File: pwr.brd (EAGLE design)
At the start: 70.3 x 58 mm, 40 parts, among them Q1 IPD65R600C6, T1 750811647, U1 UCC28700

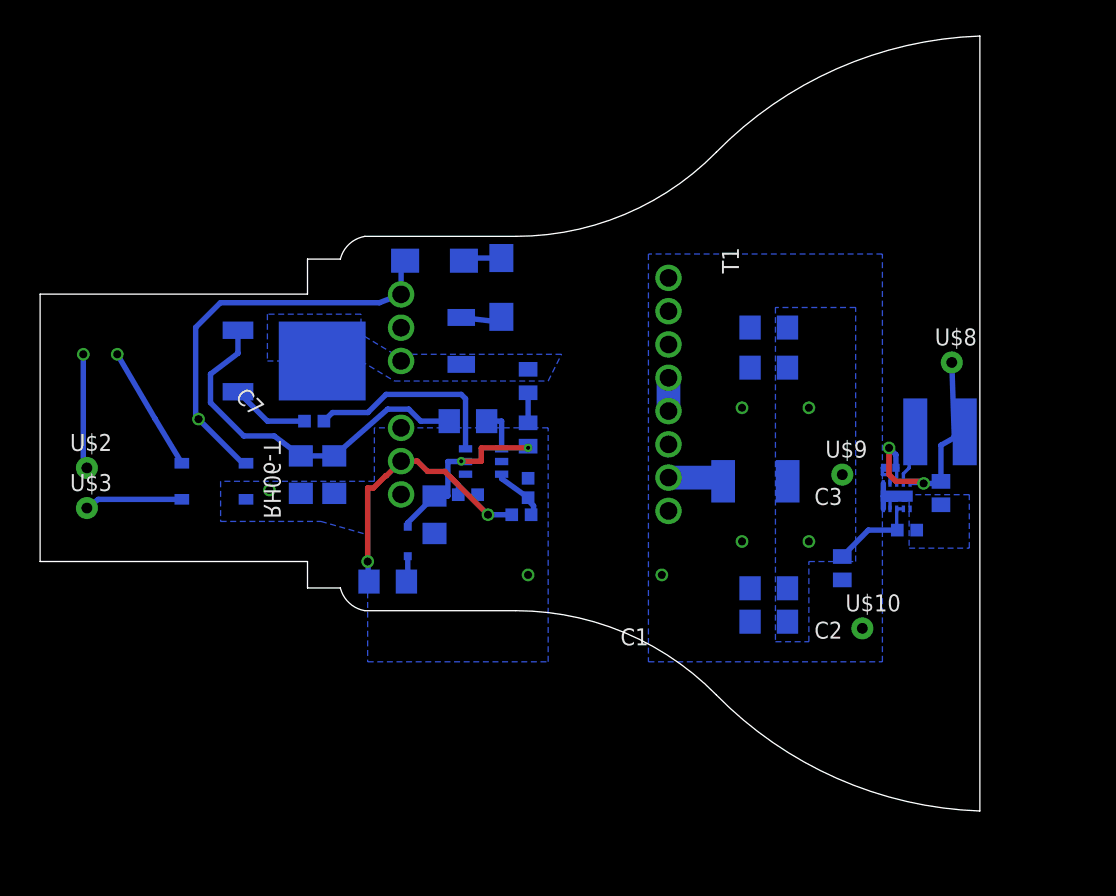
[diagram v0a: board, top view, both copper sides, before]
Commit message: save
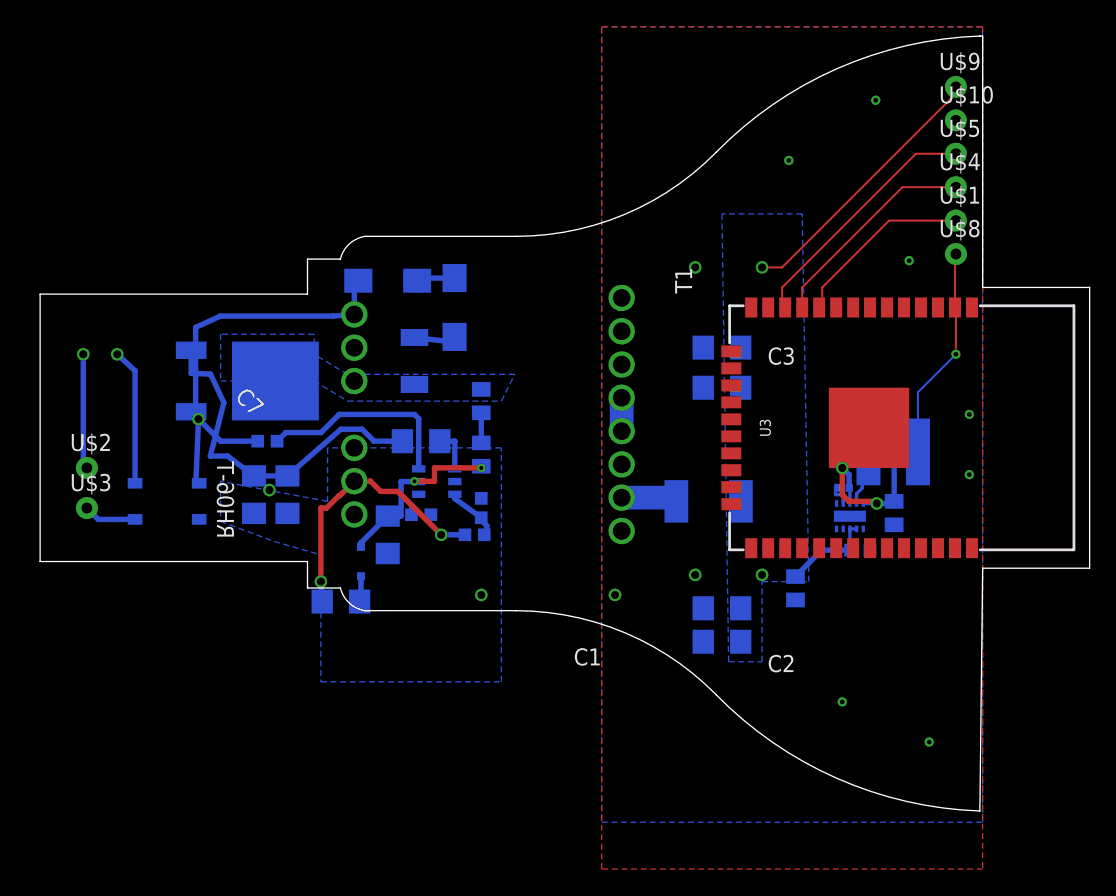
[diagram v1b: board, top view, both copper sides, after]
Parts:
- added U$1, U$4, U$5: TP-1502, derek:TP-1502
- added U3: ESP-WROOM-32, derek:ESP-WROOM-32
- moved U$10 38.6 mm to (74.0, 67.5)
- moved U$9 30.2 mm to (74.0, 70.0)
- moved C3 11.1 mm to (57.0, 56.5)
- moved U$8 8.12 mm to (74.0, 57.5)
- moved C2 4.30 mm to (57.0, 33.5)
- moved C1 3.81 mm to (43.5, 32.0)
- moved C4 3.81 mm to (56.5, 47.5)
- moved C5 3.81 mm to (56.5, 50.5)
- moved C6 3.81 mm to (62.0, 32.5)
- moved C8 3.81 mm to (34.0, 38.0)
- moved C9 3.81 mm to (31.5, 36.5)
- moved C_1 3.81 mm to (66.8, 35.4)
- moved C_2 3.81 mm to (69.4, 38.1)
- moved D1 3.81 mm to (55.5, 39.0)
- moved D2 3.81 mm to (31.5, 55.5)
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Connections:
- new net N$21: U$1.1, U3.10
- new net N$23: U$5.1, U3.12
- new net N$24: U$4.1, U3.11
- net 3.3V: now also U3.2
- net GND: now also U1.5
- net GND-ISO: now also U3.1, U3.15, U3.38, U3.GND
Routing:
- net 24V: track 7.08 -> 27.5 mm
- net N$23: track 0.00 -> 18.7 mm
- net N$24: track 0.00 -> 16.1 mm
- net N$21: track 0.00 -> 13.7 mm
- net 3.3V: track 21.2 -> 30.9 mm, vias 2 -> 3
- net GND-ISO: track 4.35 -> 0.00 mm, vias 0 -> 7
- net N$3: track 30.9 -> 26.9 mm
- net N$2: track 7.32 -> 3.95 mm
- net N$15: track 27.5 -> 26.2 mm
- net N$1: track 9.47 -> 10.2 mm
- added copper zone on layer 1, net GND-ISO
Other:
- board size 70.3 x 58 mm -> 78.5 x 58 mm

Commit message: save
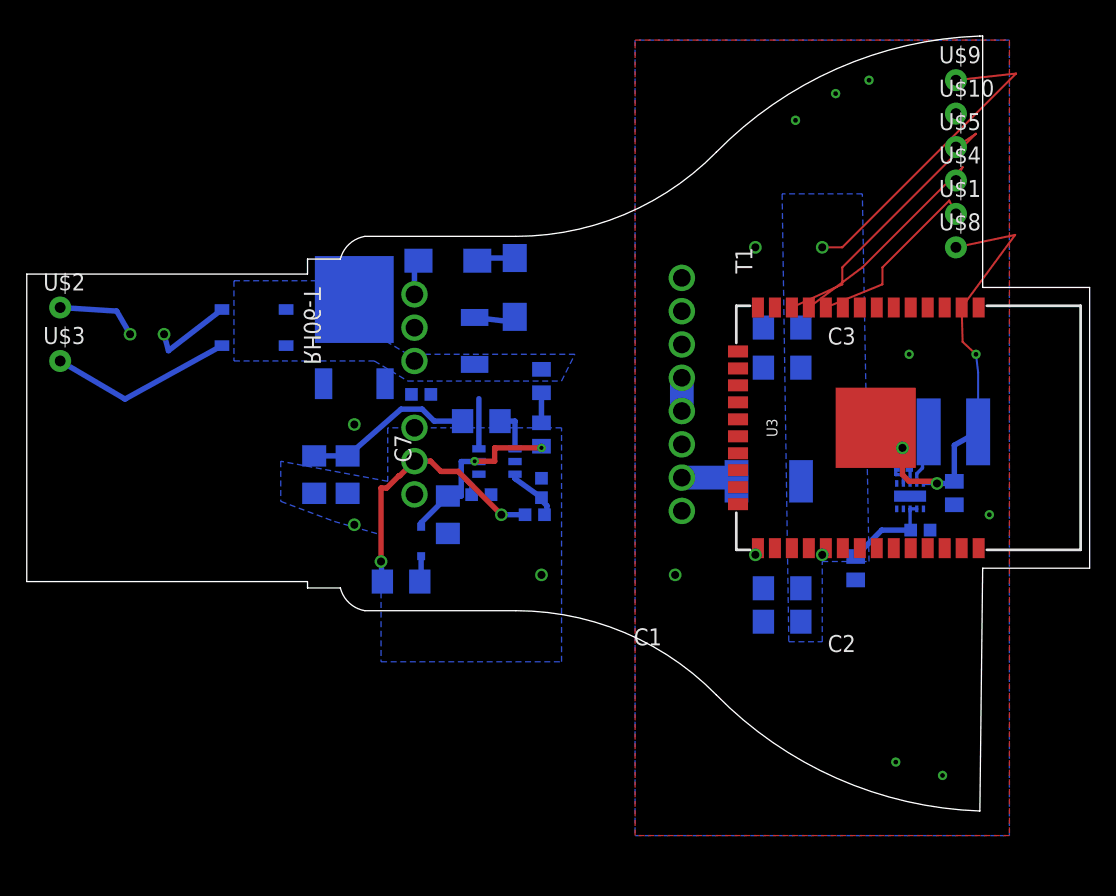
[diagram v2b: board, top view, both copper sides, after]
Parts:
- moved D3 14.5 mm to (21.5, 52.0)
- moved U$2 12.2 mm to (7.00, 53.5)
- moved R7 12.0 mm to (34.0, 47.0)
- moved U$3 11.2 mm to (7.00, 49.5)
- moved C7 9.12 mm to (29.0, 41.0), turned to 270 degrees
- moved Q1 8.94 mm to (29.0, 52.0), turned to 0 degrees
- moved C1 4.74 mm to (48.0, 33.5)
- moved C2 4.74 mm to (61.5, 35.0)
- moved C3 4.74 mm to (61.5, 58.0)
- moved C4 4.74 mm to (61.0, 49.0)
- moved C5 4.74 mm to (61.0, 52.0)
- moved C6 4.74 mm to (66.5, 34.0)
- moved C8 4.74 mm to (38.5, 39.5)
- moved C9 4.74 mm to (36.0, 38.0)
- moved C_1 4.74 mm to (71.3, 36.9)
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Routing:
- net N$3: track 26.9 -> 2.82 mm
- net N$15: track 26.2 -> 12.8 mm
- net N$13: track 15.3 -> 3.75 mm
- net N$2: track 3.95 -> 13.9 mm
- net N$12: track 5.89 -> 0.00 mm
- net 3.3V: track 30.9 -> 35.9 mm
- net 24V: track 27.5 -> 31.5 mm
- net N$1: track 10.2 -> 6.32 mm
- net N$23: track 18.7 -> 21.4 mm
- net N$11: track 8.62 -> 6.24 mm
- net N$24: track 16.1 -> 16.7 mm
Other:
- board size 78.5 x 58 mm -> 79.5 x 58 mm
